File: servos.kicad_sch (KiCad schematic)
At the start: 5 parts, among them J10 Conn_01x03_Pin, J11 Conn_01x03_Pin, J12 Conn_01x03_Pin, Q1 IPD90N04S4-05, SW2 PTS 647 SN50 SMTR2 LFS

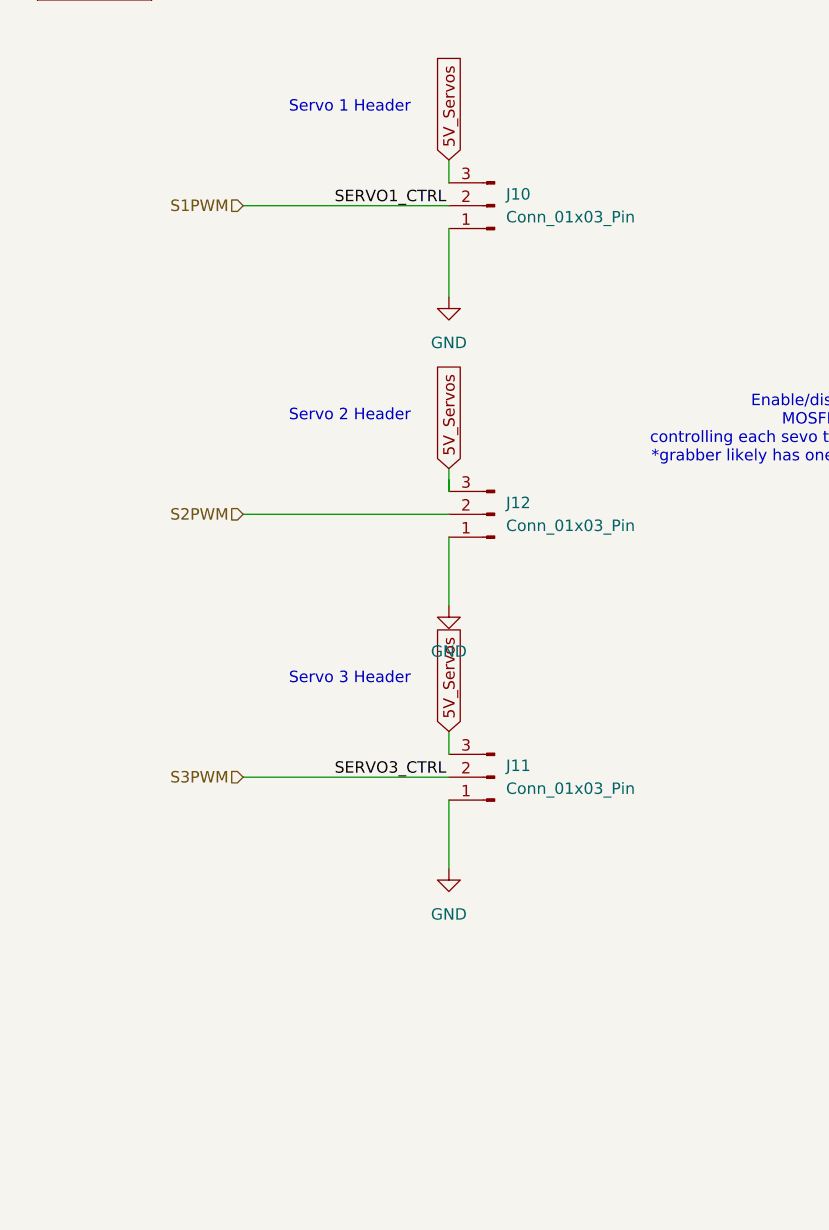
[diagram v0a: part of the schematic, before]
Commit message: updated servos with new connectors
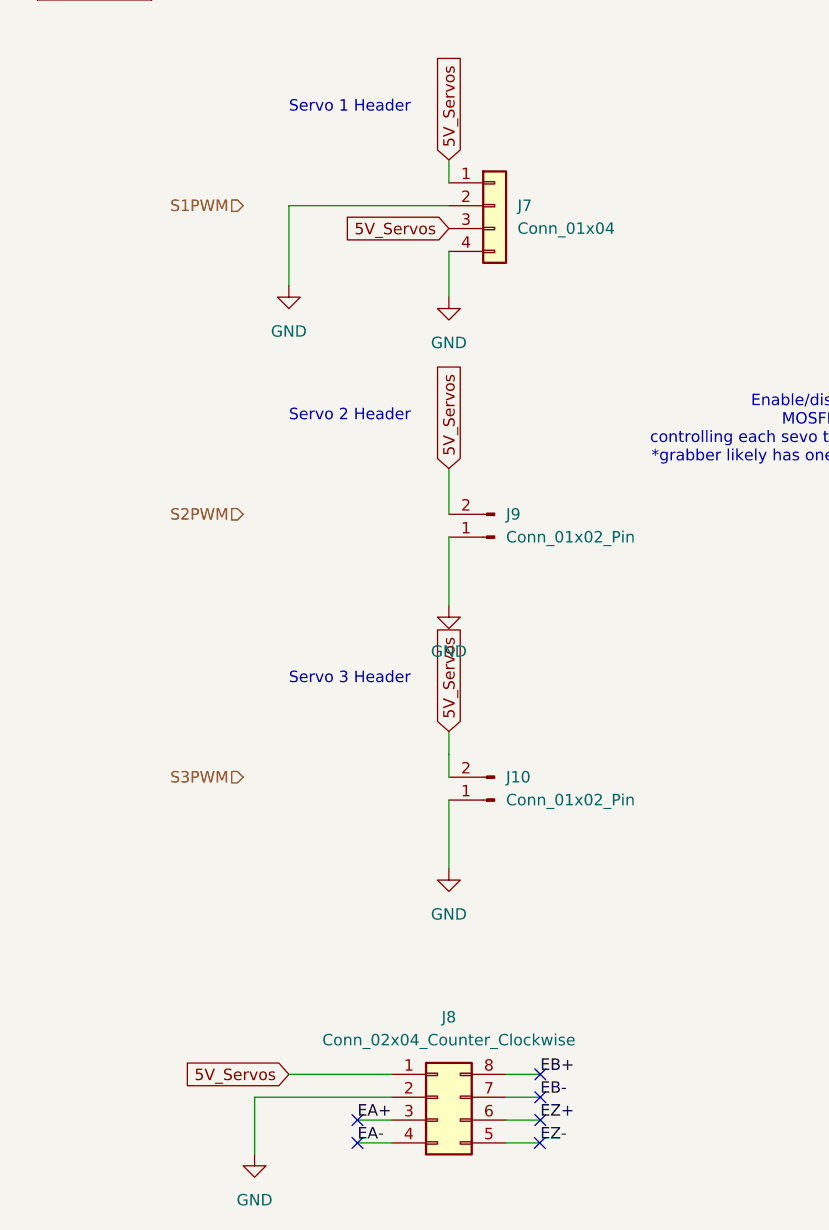
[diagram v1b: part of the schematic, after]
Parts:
- removed J10, J11, J12: Conn_01x03_Pin, Connector_PinHeader_2.54mm:PinHeader_1x03_P2.54mm_Vertical, symbol Connector:Conn_01x03_Pin
- added J10, J9: Conn_01x02_Pin, symbol Connector:Conn_01x02_Pin
- added J7: Conn_01x04, symbol Connector_Generic:Conn_01x04
- added J8: Conn_02x04_Counter_Clockwise, symbol Connector_Generic:Conn_02x04_Counter_Clockwise
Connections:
- net 5V_Servos: now also J10.2 (Pin_2), J7.1 (Pin_1), J7.3 (Pin_3), J8.1 (Pin_1), J9.2 (Pin_2)
- net GND: now also J10.1 (Pin_1), J7.2 (Pin_2), J7.4 (Pin_4), J8.2 (Pin_2), J9.1 (Pin_1)
- new net EA+: J8.3 (Pin_3)
- new net EA-: J8.4 (Pin_4)
- new net EB+: J8.8 (Pin_8)
- new net EB-: J8.7 (Pin_7)
- new net EZ+: J8.6 (Pin_6)
- new net EZ-: J8.5 (Pin_5)
- no-connect marks 1 -> 7
